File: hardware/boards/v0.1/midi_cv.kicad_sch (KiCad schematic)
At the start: 23 parts, among them J10 MIDI_OUT/THRU, J11 MIDI_IN, U19 TLP2362TPR_E, U30 TS5A23159RSE, U34 TS5A23159RSE, U35 TS5A23159RSE

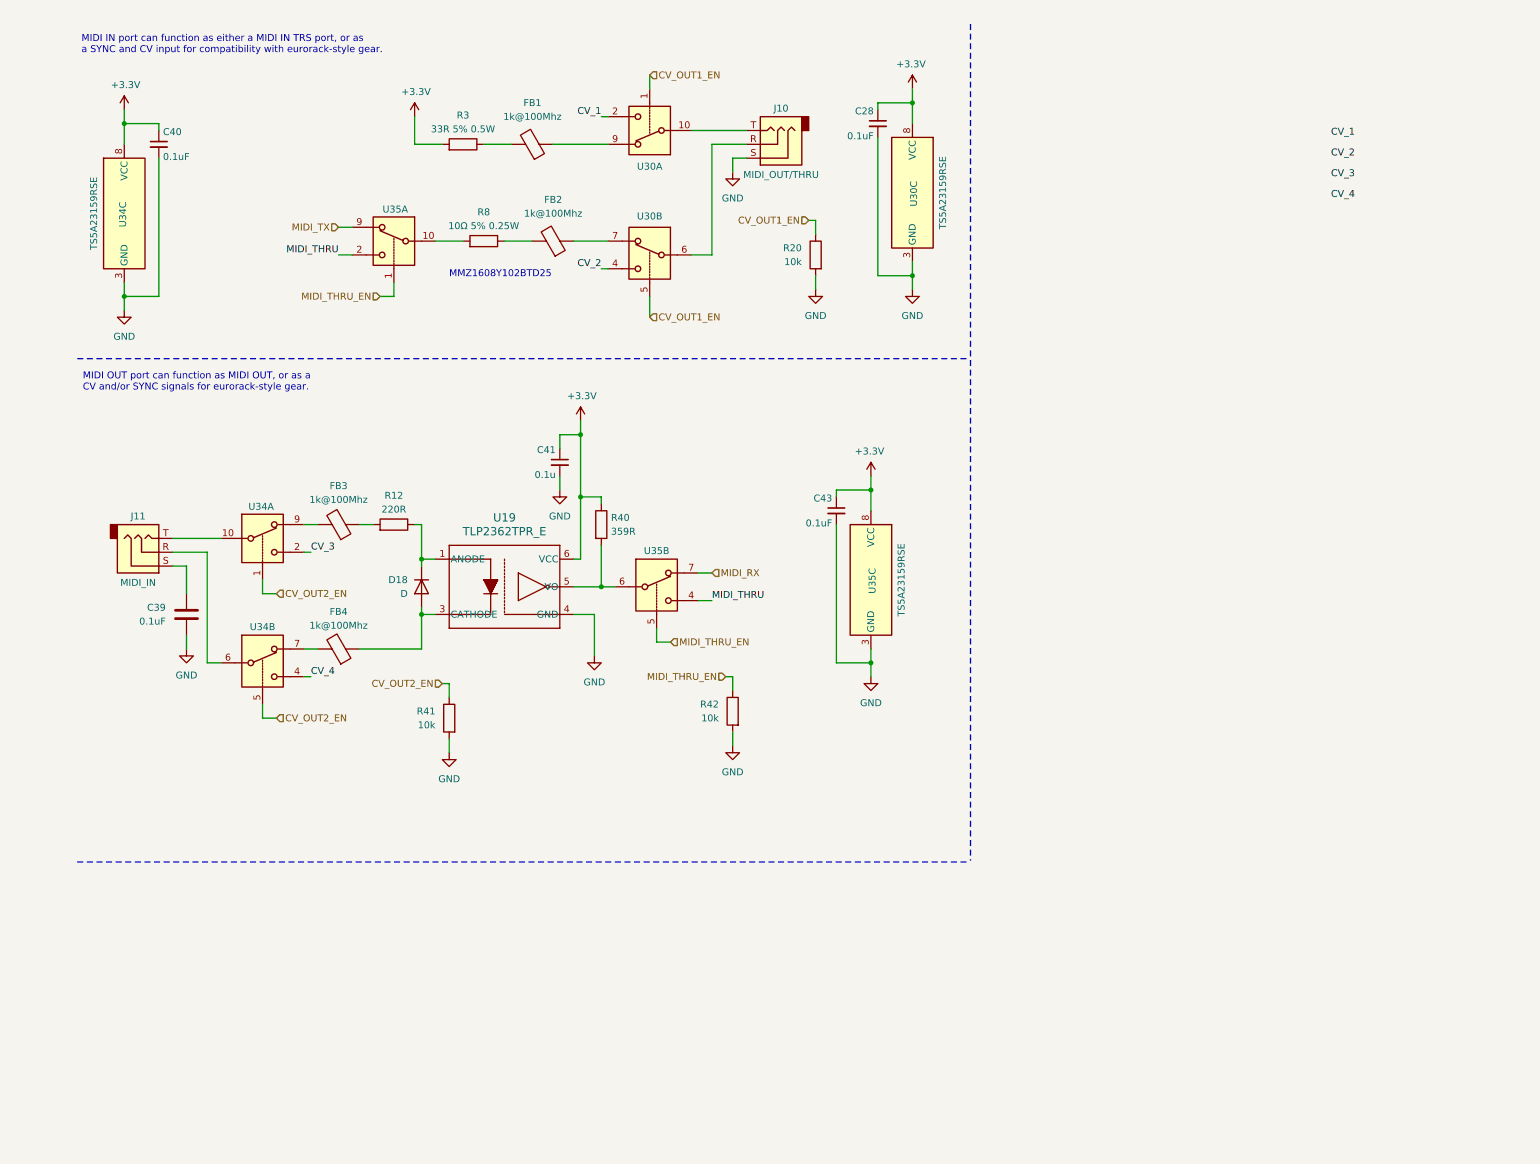
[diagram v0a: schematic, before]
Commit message: feat: various schematic organization
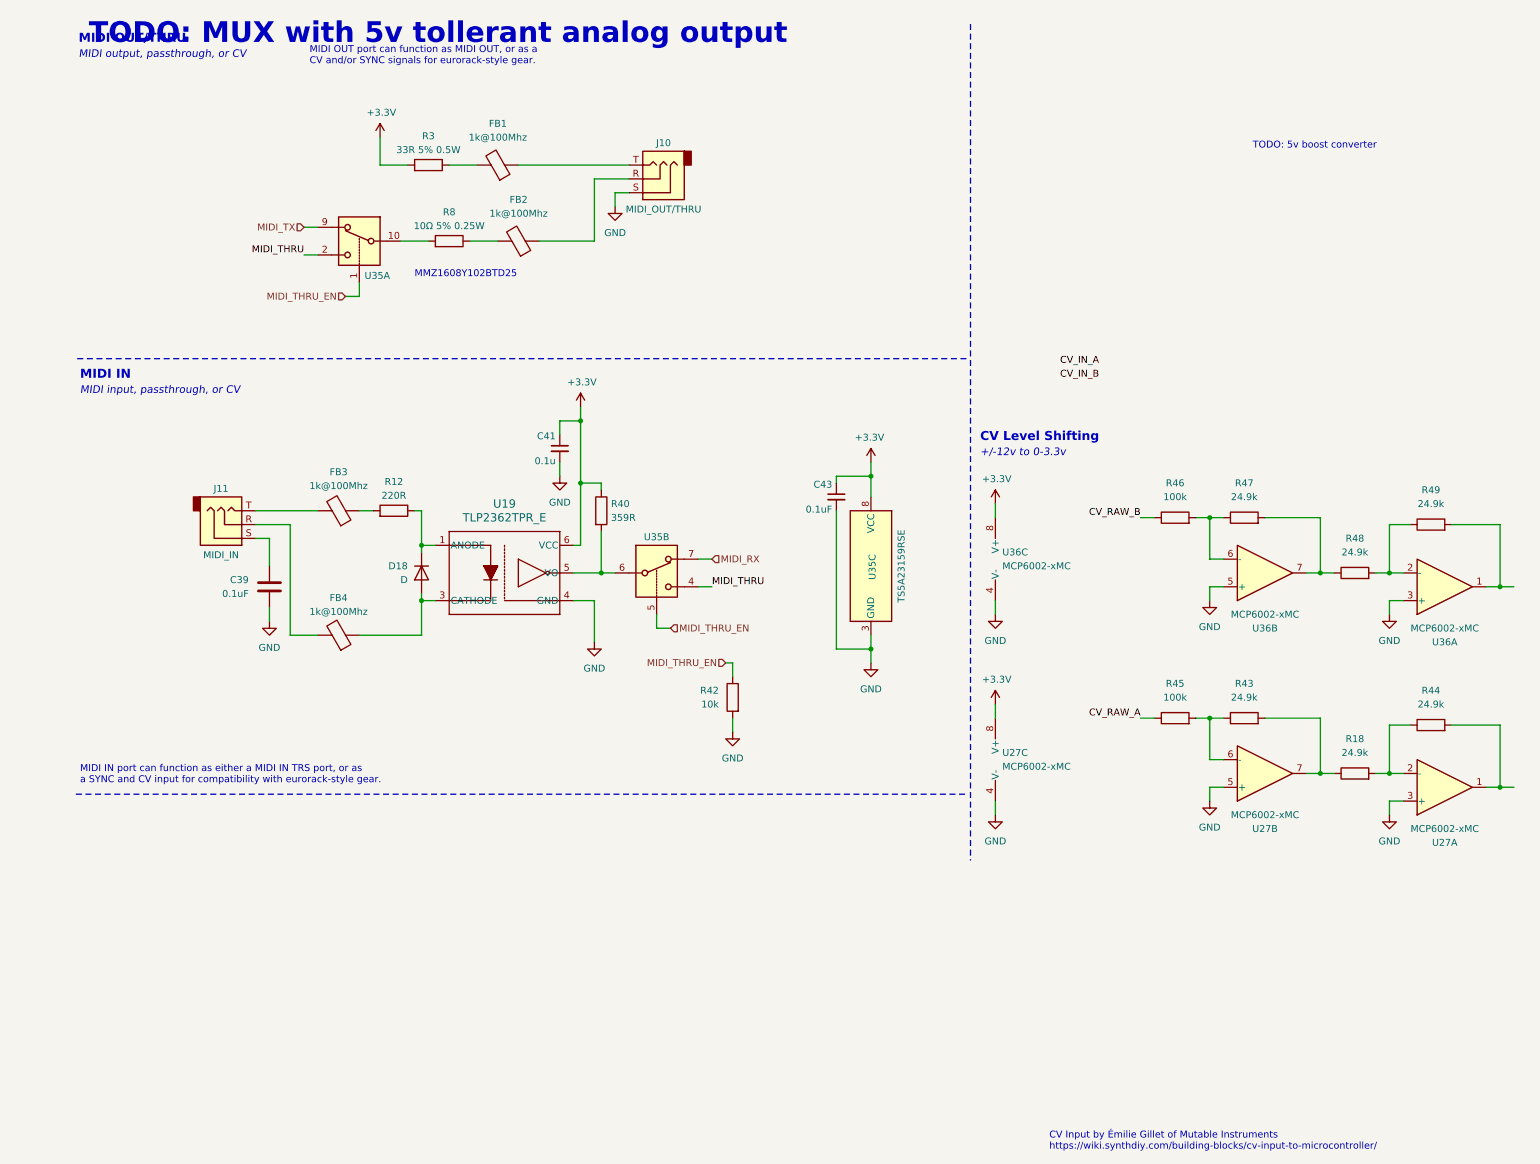
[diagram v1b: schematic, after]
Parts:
- removed C28, C40: 0.1uF, Capacitor_SMD:C_0201_0603Metric, symbol Device:C_Small
- removed R20, R41: 10k, Resistor_SMD:R_0201_0603Metric, symbol Device:R
- removed U30, U34: TS5A23159RSE, Package_DFN_QFN:Texas_R-PUQFN-N10, symbol Analog_Switch:TS5A23159RSE
- added R18, R43, R44, R47, R48, R49: 24.9k, symbol Device:R
- added R45, R46: 100k, symbol Device:R
- added U27, U36: MCP6002-xMC, Package_DFN_QFN:DFN-8-1EP_3x2mm_P0.5mm_EP1.75x1.45mm, symbol Amplifier_Operational:MCP6002-xMC
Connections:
- net +3.3V: now also U27.8 (V+), U36.8 (V+)
- net GND: now also U27.3 (+), U27.4 (V-), U27.5 (+), U27.9 (V-), U36.3 (+), U36.4 (V-), U36.5 (+), U36.9 (V-)
- net at J11.R: now also FB4.2
- net at FB3.2: now also J11.T
- net at FB2.1: now also J10.R
- net at J10.T: now also FB1.1
- new net: R43.1, R45.2, U27.6 (-)
- new net: R18.1, R43.2, U27.7
- new net: R47.2, R48.1, U36.7
- new net: R48.2, R49.1, U36.2 (-)
- new net: R18.2, R44.1, U27.2 (-)
- new net: R44.2, U27.1
- new net: R49.2, U36.1
- new net: R46.2, R47.1, U36.6 (-)
- new net CV_RAW_A: R45.1
- new net CV_RAW_B: R46.1
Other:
- note added: "+/-12v to 0-3.3v"
- note added: "CV Input by Émilie Gillet of Mutable Instruments https://wiki.synthdiy.com/building-blocks/cv-input-to-microcontroller/"
- note added: "CV Level Shifting"
- note added: "MIDI IN"
- note added: "MIDI OUT/THRU"
- note added: "MIDI input, passthrough, or CV"
- note added: "MIDI output, passthrough, or CV"
- note added: "TODO: 5v boost converter"
- note added: "TODO: MUX with 5v tollerant analog output"
- moved on the sheet: C39, C41, C43, D18, FB1, FB2, FB3, FB4, J10, J11, R12, R3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
